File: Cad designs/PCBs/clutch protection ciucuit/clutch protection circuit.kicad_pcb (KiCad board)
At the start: 2 copper layers, 68.6 x 53.3 mm, 8 parts, among them J1 Power, J2 Digital/PWM, J3 Analog, J4 Digital/PWM

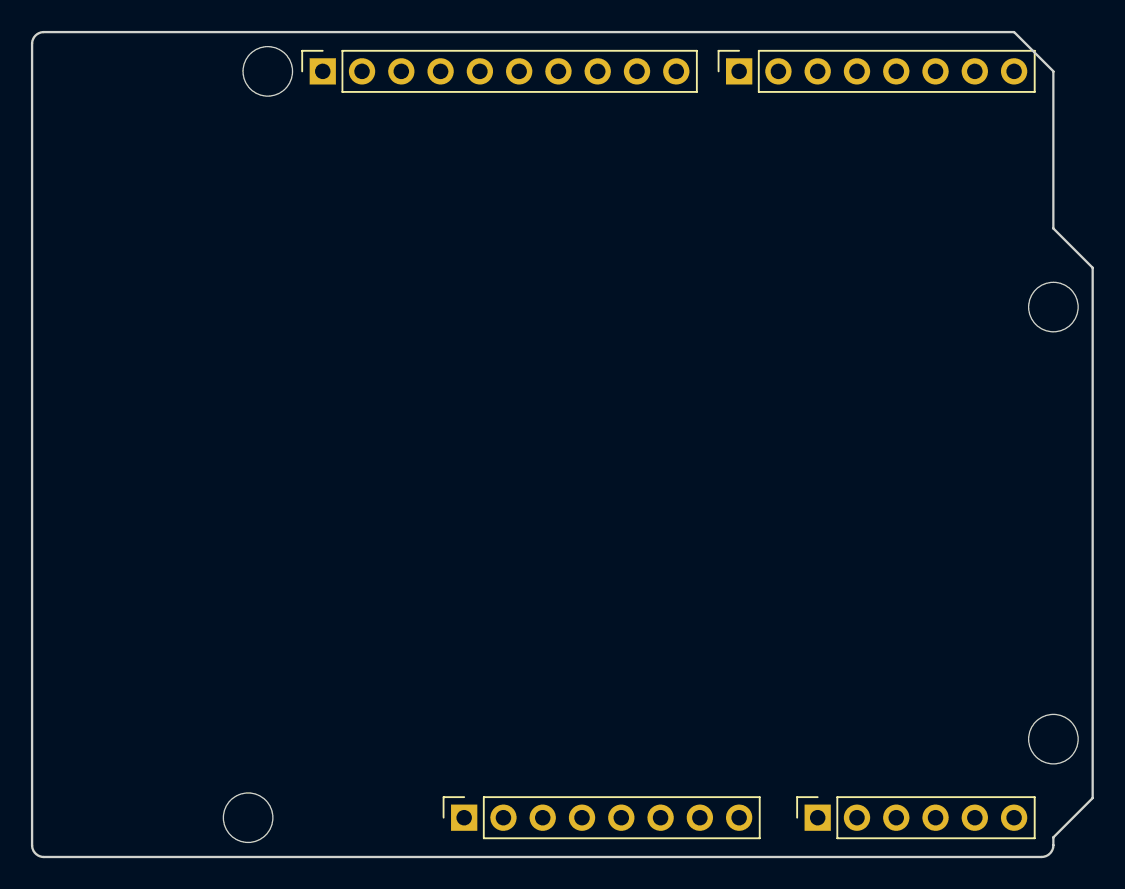
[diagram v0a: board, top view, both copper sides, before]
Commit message: 1
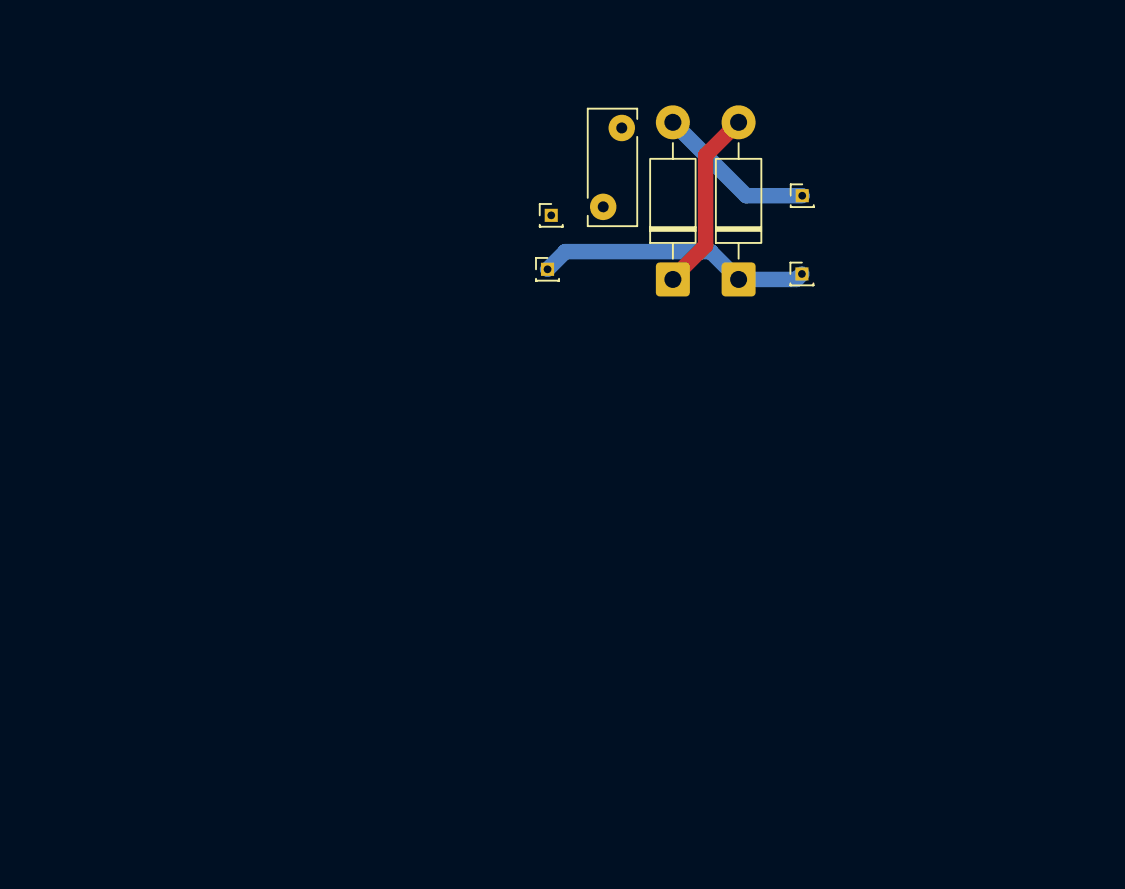
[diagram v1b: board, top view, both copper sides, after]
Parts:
- removed MH1, MH2, MH3, MH4: MountingHole_3.2mm, Arduino_MountingHole:MountingHole_3.2mm
- added D1: 1N47xxA, Diode_THT:D_DO-41_SOD81_P10.16mm_Horizontal, F.Cu at (145.7, 62.7)
- added D2: 1N5819, Diode_THT:D_DO-41_SOD81_P10.16mm_Horizontal, F.Cu at (141.4, 62.7)
- added F1: Polyfuse, Fuse:Fuse_Bourns_MF-RHT050, F.Cu at (138.1, 52.9)
- J1: value Power -> Conn_01x01; footprint Connector_PinSocket_2.54mm:PinSocket_1x08_P2.54mm_Vertical -> Connector_PinHeader_1.00mm:PinHeader_1x01_P1.00mm_Vertical
- J2: value Digital/PWM -> Conn_01x01; footprint Connector_PinSocket_2.54mm:PinSocket_1x10_P2.54mm_Vertical -> Connector_PinHeader_1.00mm:PinHeader_1x01_P1.00mm_Vertical
- J3: value Analog -> Conn_01x01; footprint Connector_PinSocket_2.54mm:PinSocket_1x06_P2.54mm_Vertical -> Connector_PinHeader_1.00mm:PinHeader_1x01_P1.00mm_Vertical
- J4: value Digital/PWM -> Conn_01x01; footprint Connector_PinSocket_2.54mm:PinSocket_1x08_P2.54mm_Vertical -> Connector_PinHeader_1.00mm:PinHeader_1x01_P1.00mm_Vertical
- moved J1 45.8 mm to (149.8, 57.2), turned to 0 degrees
- moved J3 39.5 mm to (133.3, 62.0), turned to 0 degrees
- moved J2 33.6 mm to (149.8, 62.3), turned to 0 degrees
- moved J4 15.3 mm to (133.6, 58.5), turned to 0 degrees
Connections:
- J1 pad 1: unconnected-(J1-Pin_1-Pad1) -> Net-(D2-A)
- J2 pad 1: /SCL/A5 -> Net-(D1-K)
- J3 pad 1: /A0 -> Net-(D1-K)
- J4 pad 1: /7 -> Net-(J4-Pin_1)
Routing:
- net Net-(D1-K): track 0.00 -> 17.8 mm
- net Net-(D1-A): track 0.00 -> 11.9 mm
- net Net-(D2-A): track 0.00 -> 10.7 mm
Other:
- board outline removed
- board text removed: "ICSP"
